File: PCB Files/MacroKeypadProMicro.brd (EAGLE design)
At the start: 61 x 62.2 mm, 8 parts

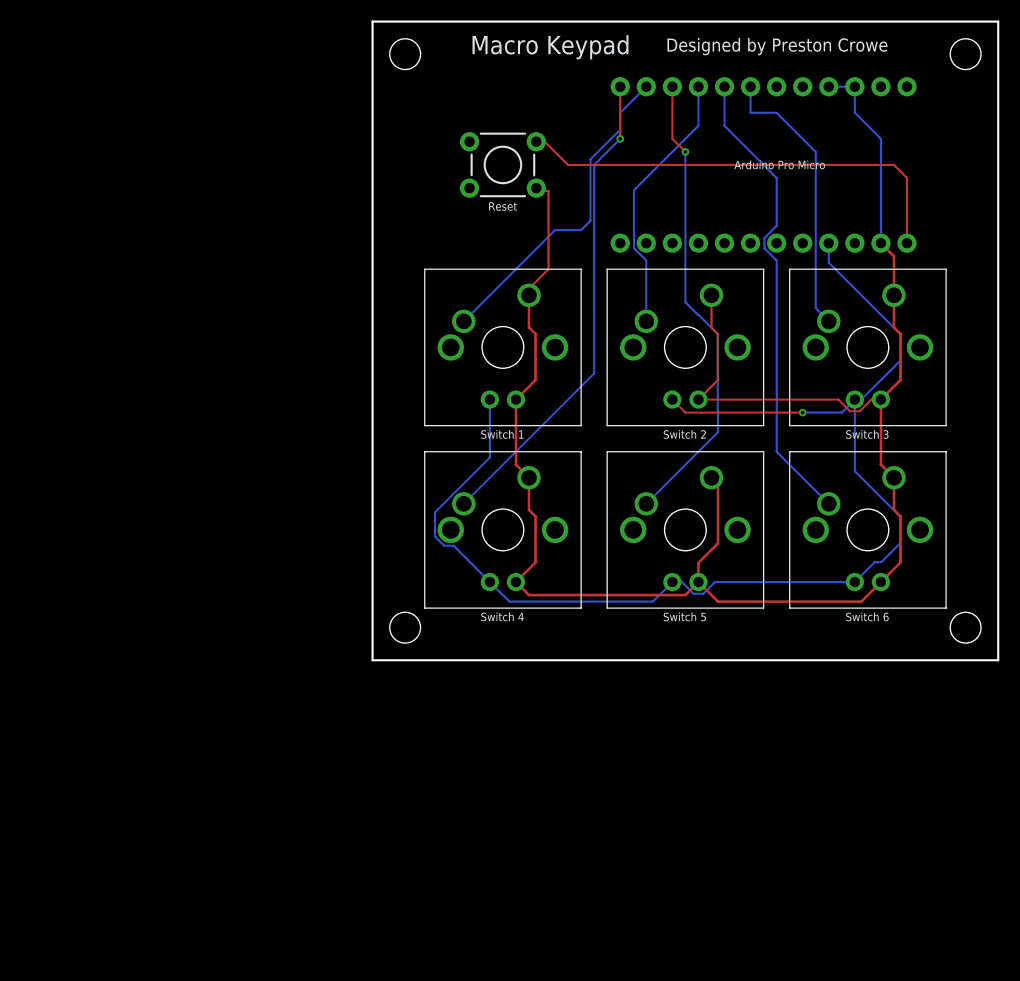
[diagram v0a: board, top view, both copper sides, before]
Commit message: Finished updated Pro Micro board
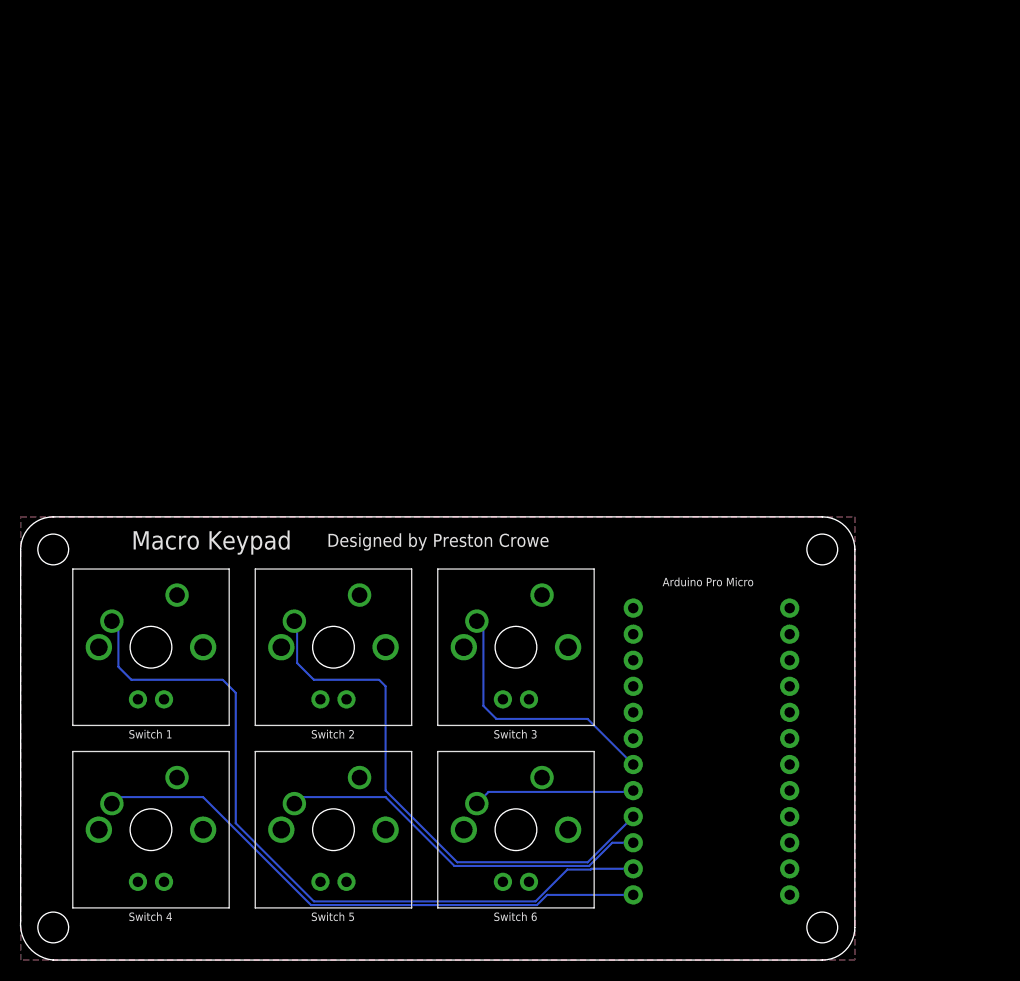
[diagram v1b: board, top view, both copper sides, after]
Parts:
- removed S1: MOMENTARY-SWITCH-SPST-PTH-6.0MM, SparkFun-Switches:TACTILE_SWITCH_PTH_6.0MM
- moved B1 56.2 mm to (67.3, 21.6), turned to 0 degrees
- moved U$1 45.0 mm to (12.7, 12.7)
- moved U$7 45.0 mm to (12.7, 30.5)
- moved U$4 45.0 mm to (48.3, 30.5)
- moved U$5 45.0 mm to (48.3, 12.7)
- moved U$2 45.0 mm to (30.5, 12.7)
- moved U$3 45.0 mm to (30.5, 30.5)
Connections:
- removed net LED+: B1.20, B1.21, U$1.LED+, U$2.LED+, U$3.LED+, U$4.LED+, U$5.LED+, U$7.LED+
- removed net RESET: B1.24, S1.3
- new net N$2: B1.20, B1.21
- new net RAW: B1.24
- net GND: no longer S1.1, U$1.LED-, U$2.LED-, U$3.LED-, U$4.LED-, U$5.LED-, U$7.LED-
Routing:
- net GND: track 177.2 -> 0.00 mm
- net LED+: track 121.8 -> 0.00 mm, vias 1 -> 0
- net RESET: track 44.2 -> 0.00 mm
- net SW1: track 31.7 -> 73.1 mm
- net SW6: track 45.8 -> 15.9 mm
- net SW2: track 26.0 -> 52.8 mm
- net SW4: track 47.0 -> 55.8 mm, vias 1 -> 0
- net SW5: track 45.4 -> 37.0 mm, vias 1 -> 0
- net SW3: track 27.5 -> 25.5 mm
- added copper zone on layer 1, net GND
- added copper zone on layer 16, net GND
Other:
- board size 61 x 62.2 mm -> 81.3 x 43.2 mm
- board text added: "github.com/vaugerbird/Macro-Keypad"
- board text removed: "Reset"
- board text removed: "Rev 1 - L/B"
- board text removed: "github.com/PrestonCrowe/Macro-Keypad"
